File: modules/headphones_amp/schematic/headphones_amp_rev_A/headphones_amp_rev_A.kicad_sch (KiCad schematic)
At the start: 24 parts, among them Q1 BC140, Q2 BC160, Q3 BC548, Q4 BC557, Q5 BC548, Q6 BC548

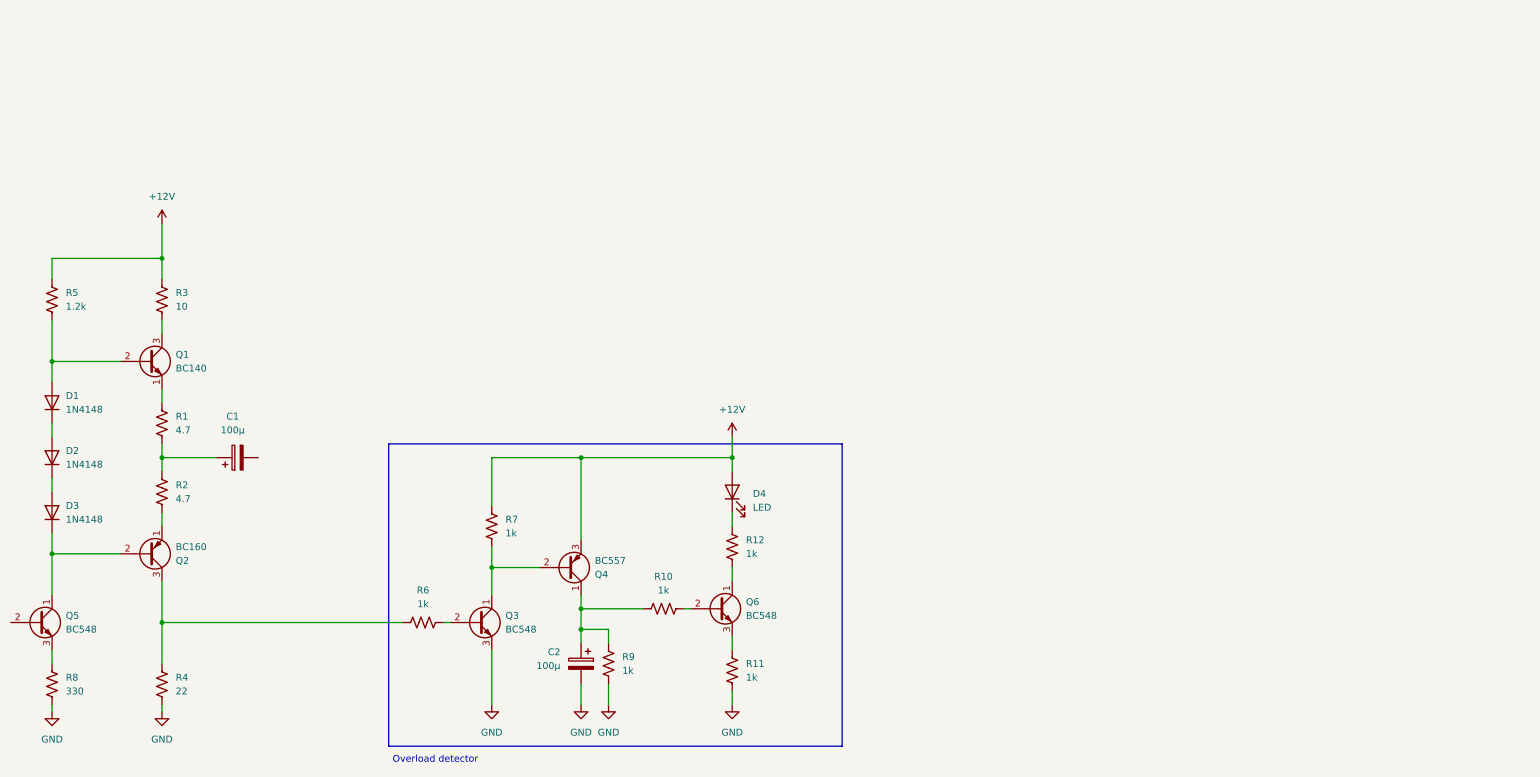
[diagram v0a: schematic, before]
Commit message: added new references to the PPL
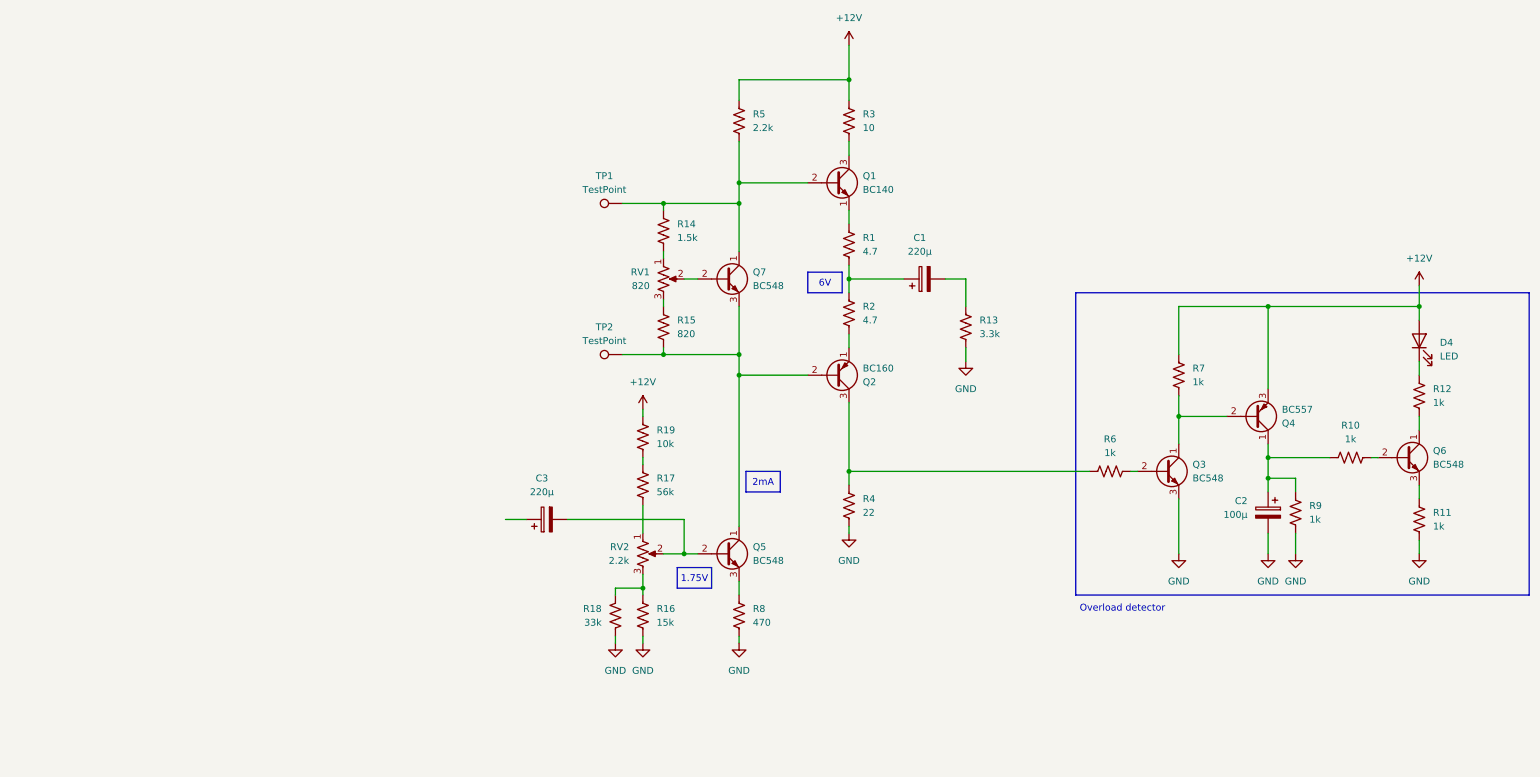
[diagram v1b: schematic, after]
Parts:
- removed D1, D2, D3: 1N4148, Diode_THT:D_DO-35_SOD27_P7.62mm_Horizontal, symbol Diode:1N4148
- added C3: 220µ, Capacitor_THT:CP_Radial_D10.0mm_P5.00mm, symbol Device:C_Polarized
- added Q7: BC548, Package_TO_SOT_THT:TO-92L_Inline_Wide, symbol Transistor_BJT:BC548
- added R13: 3.3k, Resistor_THT:R_Axial_DIN0207_L6.3mm_D2.5mm_P10.16mm_Horizontal, symbol Device:R_US
- added R14: 1.5k, Resistor_THT:R_Axial_DIN0207_L6.3mm_D2.5mm_P10.16mm_Horizontal, symbol Device:R_US
- added R15: 820, Resistor_THT:R_Axial_DIN0207_L6.3mm_D2.5mm_P10.16mm_Horizontal, symbol Device:R_US
- added R16: 15k, Resistor_THT:R_Axial_DIN0207_L6.3mm_D2.5mm_P10.16mm_Horizontal, symbol Device:R_US
- added R17: 56k, Resistor_THT:R_Axial_DIN0207_L6.3mm_D2.5mm_P10.16mm_Horizontal, symbol Device:R_US
- added R18: 33k, Resistor_THT:R_Axial_DIN0207_L6.3mm_D2.5mm_P10.16mm_Horizontal, symbol Device:R_US
- added R19: 10k, Resistor_THT:R_Axial_DIN0207_L6.3mm_D2.5mm_P10.16mm_Horizontal, symbol Device:R_US
- added RV1: 820, Potentiometer_THT:Potentiometer_Bourns_3296W_Vertical, symbol Device:R_Potentiometer_US
- added RV2: 2.2k, Potentiometer_THT:Potentiometer_Bourns_3296W_Vertical, symbol Device:R_Potentiometer_US
- added TP1, TP2: TestPoint, TestPoint:TestPoint_Pad_D2.0mm, symbol Connector:TestPoint
- C1: value 100µ -> 220µ
- R5: value 1.2k -> 2.2k
- R8: value 330 -> 470
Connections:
- net +12V: now also R19.2
- net GND: now also R13.2, R16.2, R18.2
- net at Q1.2 (B), R5.2: now also Q7.1 (C), R14.1, TP1.1
- net at C1.2: now also R13.1
- net at Q2.2 (B), Q5.1 (C): now also Q7.3 (E), R15.2, TP2.1
- net at Q5.2 (B): now also C3.2, RV2.2
- new net: R17.1, R19.1
- new net: R17.2, RV2.1
- new net: R16.1, R18.1, RV2.3
- new net: R15.1, RV1.3
- new net: R14.2, RV1.1
- new net: Q7.2 (B), RV1.2
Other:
- moved on the sheet: C1, C2, D4, Q1, Q2, Q3, Q4, Q5, Q6, R1, R10, R11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
